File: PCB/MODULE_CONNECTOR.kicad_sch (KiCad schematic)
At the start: 1 part, among them J4 Conn_02x20_Odd_Even

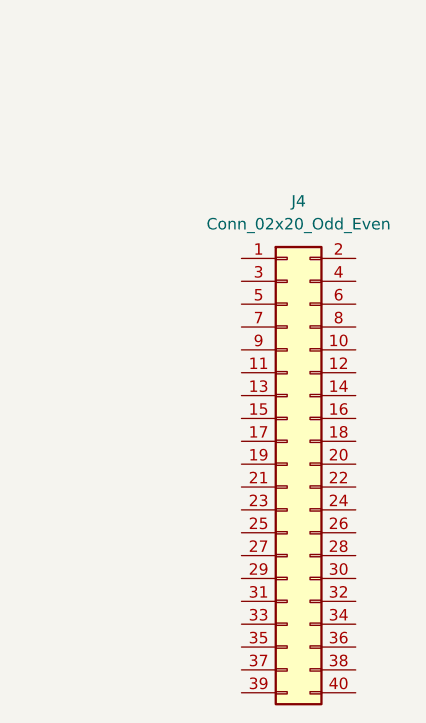
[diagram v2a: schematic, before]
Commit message: PCB_UPDATE
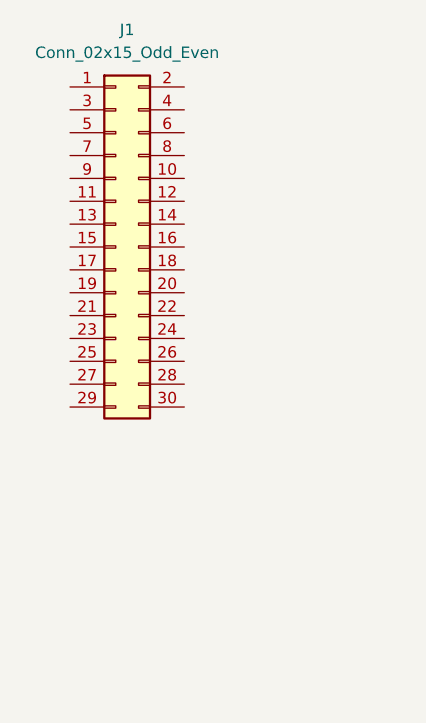
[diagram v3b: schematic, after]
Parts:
- removed J4: Conn_02x20_Odd_Even, Connector_PinHeader_1.27mm:PinHeader_2x20_P1.27mm_Horizontal, symbol Connector_Generic:Conn_02x20_Odd_Even
- added J1: Conn_02x15_Odd_Even, Connector_PinHeader_2.54mm:PinHeader_2x15_P2.54mm_Horizontal, symbol Connector_Generic:Conn_02x15_Odd_Even
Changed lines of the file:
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@@
 	(paper "A4")
 	(symbol
-		(lib_id "Connector_Generic:Conn_02x20_Odd_Even")
-		(at 146.05 104.14 0)
+		(lib_id "Connector_Generic:Conn_02x15_Odd_Even")
+		(at 127 80.01 0)
 		(unit 1)
 		(exclude_from_sim no)
@@
 		(dnp no)
 		(fields_autoplaced yes)
-		(property "Reference" "J4"
-			(at 147.32 74.93 0)
+		(property "Reference" "J1"
+			(at 128.27 55.88 0)
 			(effects
 				(font
@@
 			)
 		)
-		(property "Value" "Conn_02x20_Odd_Even"
-			(at 147.32 77.47 0)
+		(property "Value" "Conn_02x15_Odd_Even"
+			(at 128.27 58.42 0)
 			(effects
 				(font
@@
 			)
 		)
-		(property "Footprint" "Connector_PinHeader_1.27mm:PinHeader_2x20_P1.27mm_Horizontal"
-			(at 146.05 104.14 0)
+		(property "Footprint" "Connector_PinHeader_2.54mm:PinHeader_2x15_P2.54mm_Horizontal"
+			(at 127 80.01 0)
 			(effects
 				(font
@@
 		)
 		(property "Datasheet" "~"
-			(at 146.05 104.14 0)
+			(at 127 80.01 0)
 			(effects
 				(font
@@
 			)
 		)
-		(property "Description" "Generic connector, double row, 02x20, odd/even pin numbering scheme (row 1 odd numbers, row 2 even numbers), script generated (kicad-library-utils/schlib/autogen/connector/)"
-			(at 146.05 104.14 0)
+		(property "Description" "Generic connector, double row, 02x15, odd/even pin numbering scheme (row 1 odd numbers, row 2 even numbers), script generated (kicad-library-utils/schlib/autogen/connector/)"
+			(at 127 80.01 0)
 			(effects
 				(font
@@
 			)
 		)
-		(pin "9"
+		(pin "1"
 		)
-		(pin "19"
-		)
-		(pin "1"
+		(pin "5"
 		)
 		(pin "3"
 		)
-		(pin "5"
-		)
 		(pin "7"
 		)
-		(pin "11"
-		)
-		(pin "13"
-		)
-		(pin "15"
-		)
-		(pin "17"
-		)
-		(pin "21"
-		)
-		(pin "23"
-		)
-		(pin "25"
-		)
 		(pin "18"
-		)
-		(pin "35"
-		)
-		(pin "29"
-		)
-		(pin "37"
-		)
-		(pin "39"
-		)
-		(pin "2"
-		)
-		(pin "33"
-		)
-		(pin "22"
-		)
-		(pin "40"
-		)
-		(pin "20"
-		)
-		(pin "14"
-		)
-		(pin "36"
-		)
-		(pin "31"
-		)
-		(pin "4"
-		)
-		(pin "10"
-		)
-		(pin "24"
 		)
 		(pin "16"
@@
 		(pin "26"
 		)
-		(pin "32"
+		(pin "29"
+		)
+		(pin "2"
+		)
+		(pin "8"
+		)
+		(pin "9"
+		)
+		(pin "17"
+		)
+		(pin "11"
+		)
+		(pin "4"
+		)
+		(pin "14"
+		)
+		(pin "15"
+		)
+		(pin "25"
 		)
 		(pin "6"
 		)
-		(pin "34"
+		(pin "20"
+		)
+		(pin "27"
+		)
+		(pin "24"
+		)
+		(pin "22"
 		)
 		(pin "30"
 		)
-		(pin "38"
+		(pin "19"
 		)
-		(pin "28"
+		(pin "13"
+		)
+		(pin "21"
+		)
+		(pin "10"
 		)
 		(pin "12"
 		)
-		(pin "27"
+		(pin "23"
 		)
-		(pin "8"
+		(pin "28"
 		)
 		(instances
 			(project ""
 				(path "/65890f61-d586-475b-928a-b635a5e4e59e/ba2dc7bc-21cc-4648-b7c2-5eb24b24edf1"
-					(reference "J4")
+					(reference "J1")
 					(unit 1)
 				)

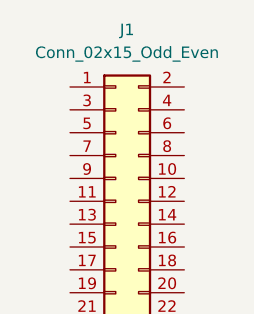
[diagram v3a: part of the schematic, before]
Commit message: PCB_UPDATE
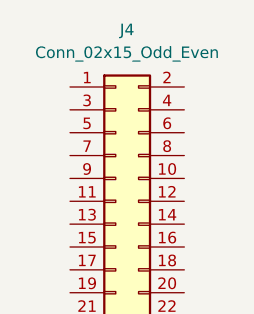
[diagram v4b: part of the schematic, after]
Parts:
- renumbered J1 to J4
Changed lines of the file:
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@@
 		(dnp no)
 		(fields_autoplaced yes)
-		(property "Reference" "J1"
+		(property "Reference" "J4"
 			(at 128.27 55.88 0)
 			(effects
@@
 			(project ""
 				(path "/65890f61-d586-475b-928a-b635a5e4e59e/ba2dc7bc-21cc-4648-b7c2-5eb24b24edf1"
-					(reference "J1")
+					(reference "J4")
 					(unit 1)
 				)
